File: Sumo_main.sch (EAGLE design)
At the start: 25 parts, among them U1 ATMEGA8U2AU, X1 MINI-USB-SCHIELD-32005-201, X2 ESC1, X3 ESC2, X4 IR Sensor 1, X5 IR Sensor 2, X6 IR Sensor 3, Y1 4MHz

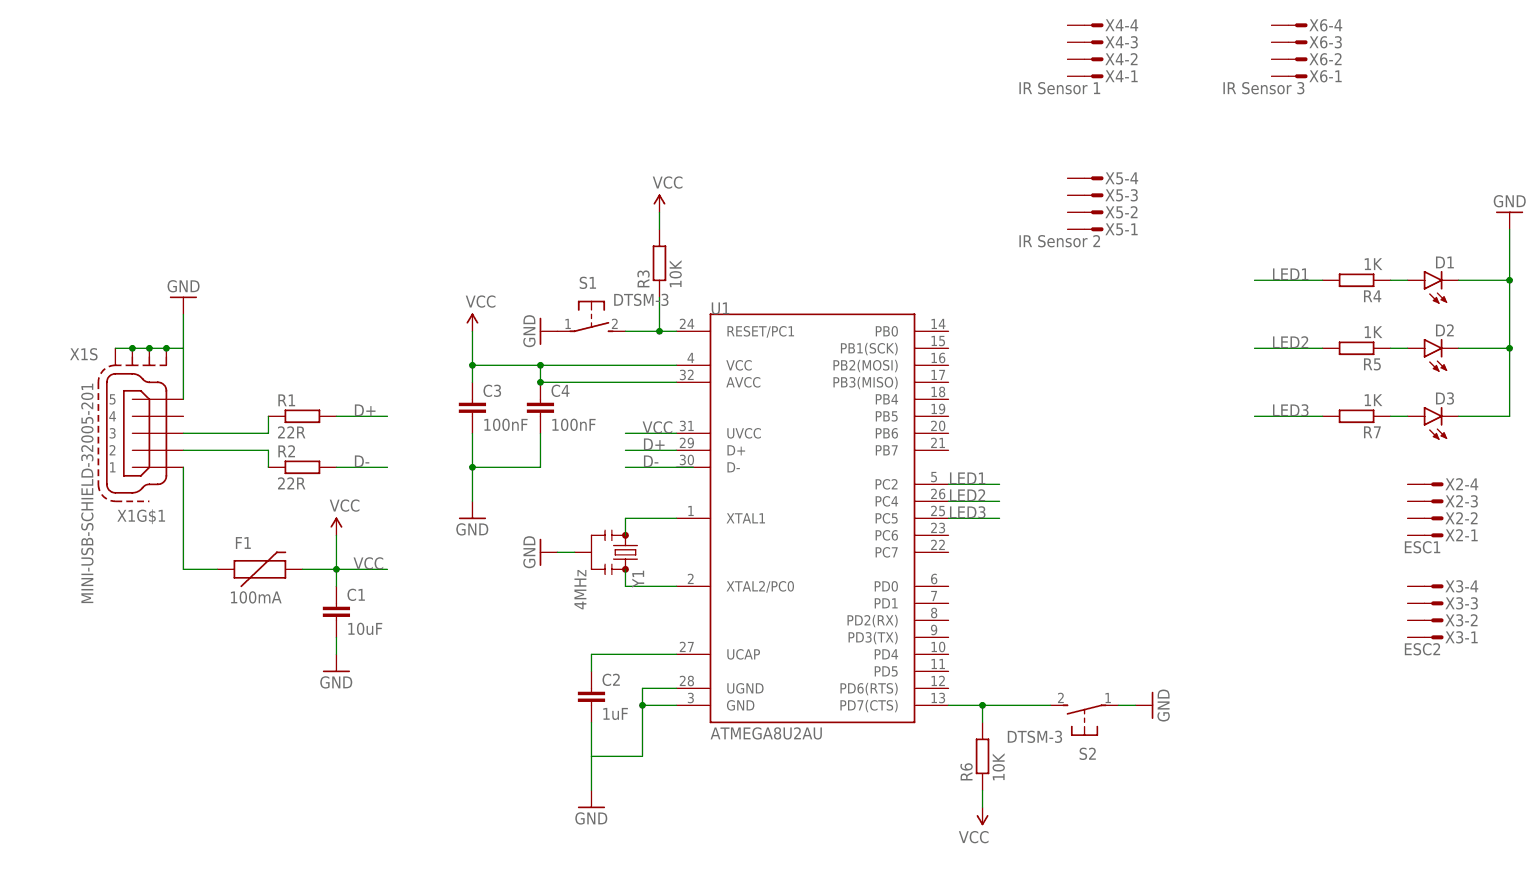
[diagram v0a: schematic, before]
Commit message: Added RS-485
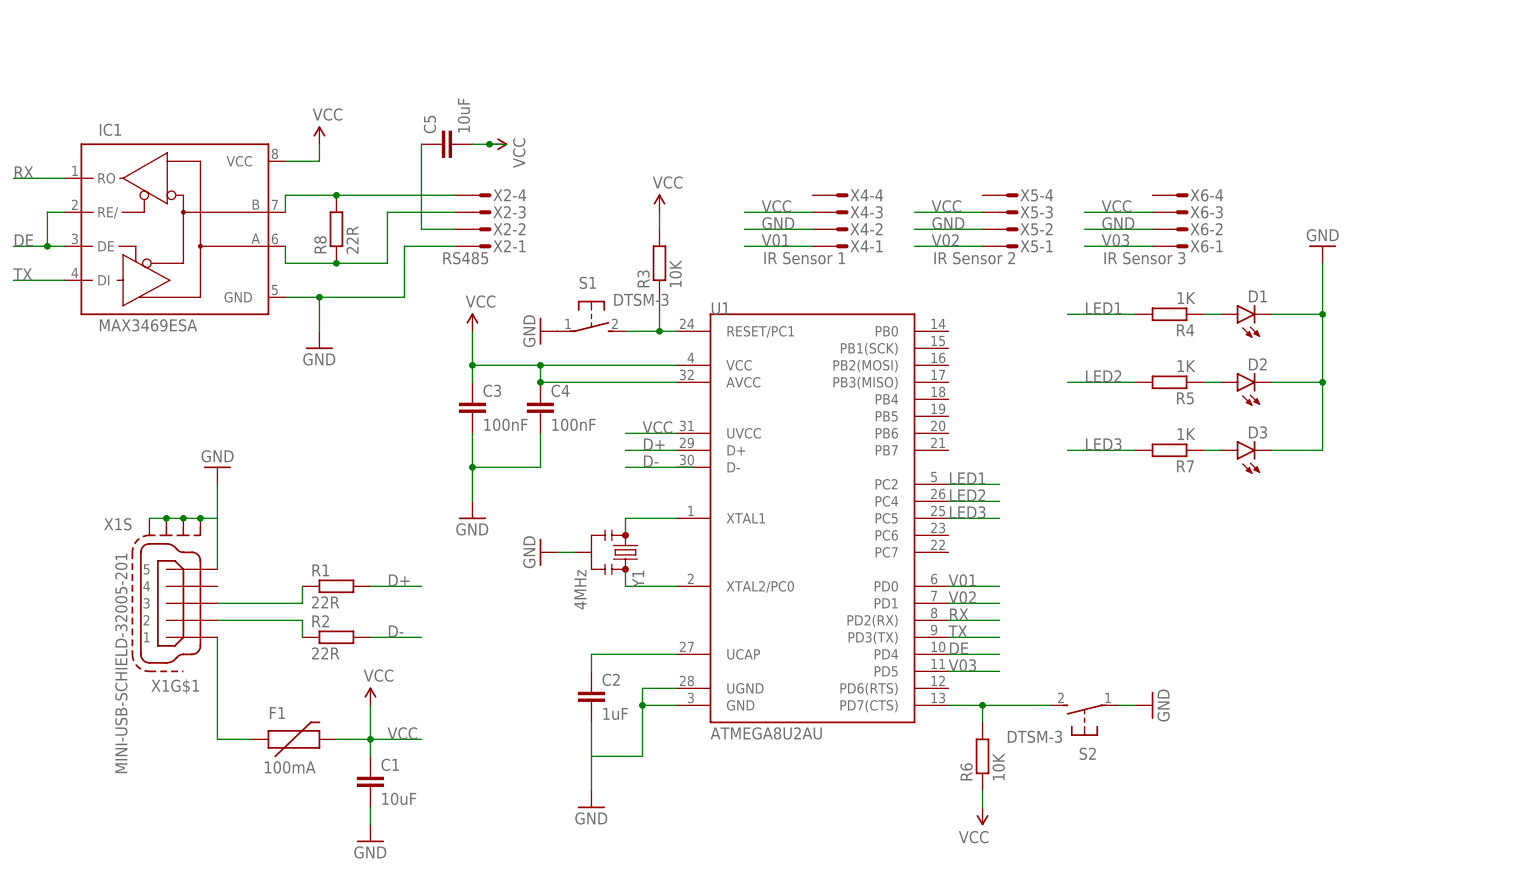
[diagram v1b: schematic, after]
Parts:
- removed X3: ESC2, con-amp-micromatch:MICROMATCH-4
- added C5: 10uF, SparkFun-Capacitors:CAP0603-CAP
- added IC1: MAX3469ESA, maxim:MAX3469ESA
- added R8: 22R, resistor:R-EU_R0603
- X2: value ESC1 -> RS485
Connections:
- new net DE: IC1.DE, IC1.RE/, U1.PD4
- new net N$11: IC1.B, R8.2, X2-4.S
- new net N$12: IC1.A, R8.1, X2-3.S
- new net N$15: C5.1, X2-2.S
- new net RX: IC1.RO, U1.PD2(RX)
- new net TX: IC1.DI, U1.PD3(TX)
- new net V01: U1.PD0, X4-1.S
- new net V02: U1.PD1, X5-1.S
- new net V03: U1.PD5, X6-1.S
- net GND: now also IC1.GND, X2-1.S, X4-2.S, X5-2.S, X6-2.S
- net VCC: now also C5.2, IC1.VCC, X4-3.S, X5-3.S, X6-3.S
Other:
- moved on the sheet: C1, D1, D2, D3, F1, R1, R2, R4, R5, R7, X1G$1, X1S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
